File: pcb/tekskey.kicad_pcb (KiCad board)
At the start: 2 copper layers, 128.6 x 128.6 mm, 124 parts, among them J1 Conn_01x08, J2 Conn_01x08, SW0 MX_SW_HS, SW1 MX_SW_HS, SW10 MX_SW_HS, SW11 MX_SW_HS, SW12 MX_SW_HS, SW13 MX_SW_HS, SW14 MX_SW_HS, SW15 MX_SW_HS, SW1B1 MX_SW_HS, SW2 MX_SW_HS, SW20 MX_SW_HS, SW21 MX_SW_HS, SW22 MX_SW_HS, SW23 MX_SW_HS, SW24 MX_SW_HS, SW25 MX_SW_HS, SW2B1 MX_SW_HS, SW3 MX_SW_HS, SW30 MX_SW_HS, SW31 MX_SW_HS, SW32 MX_SW_HS, SW33 MX_SW_HS, SW34 MX_SW_HS, SW35 MX_SW_HS, SW3B1 MX_SW_HS, SW4 MX_SW_HS, SW40 MX_SW_HS, SW41 MX_SW_HS, SW42 MX_SW_HS, SW43 MX_SW_HS, SW44 MX_SW_HS, SW45 MX_SW_HS, SW4B1 MX_SW_HS, SW5 MX_SW_HS, SW50 MX_SW_HS, SW51 MX_SW_HS, SW51B1 MX_SW_HS, SW52 MX_SW_HS, SW53 MX_SW_HS, SW54 MX_SW_HS, SW55 MX_SW_HS, SW55B1 MX_SW_HS, SW5B1 MX_SW_HS

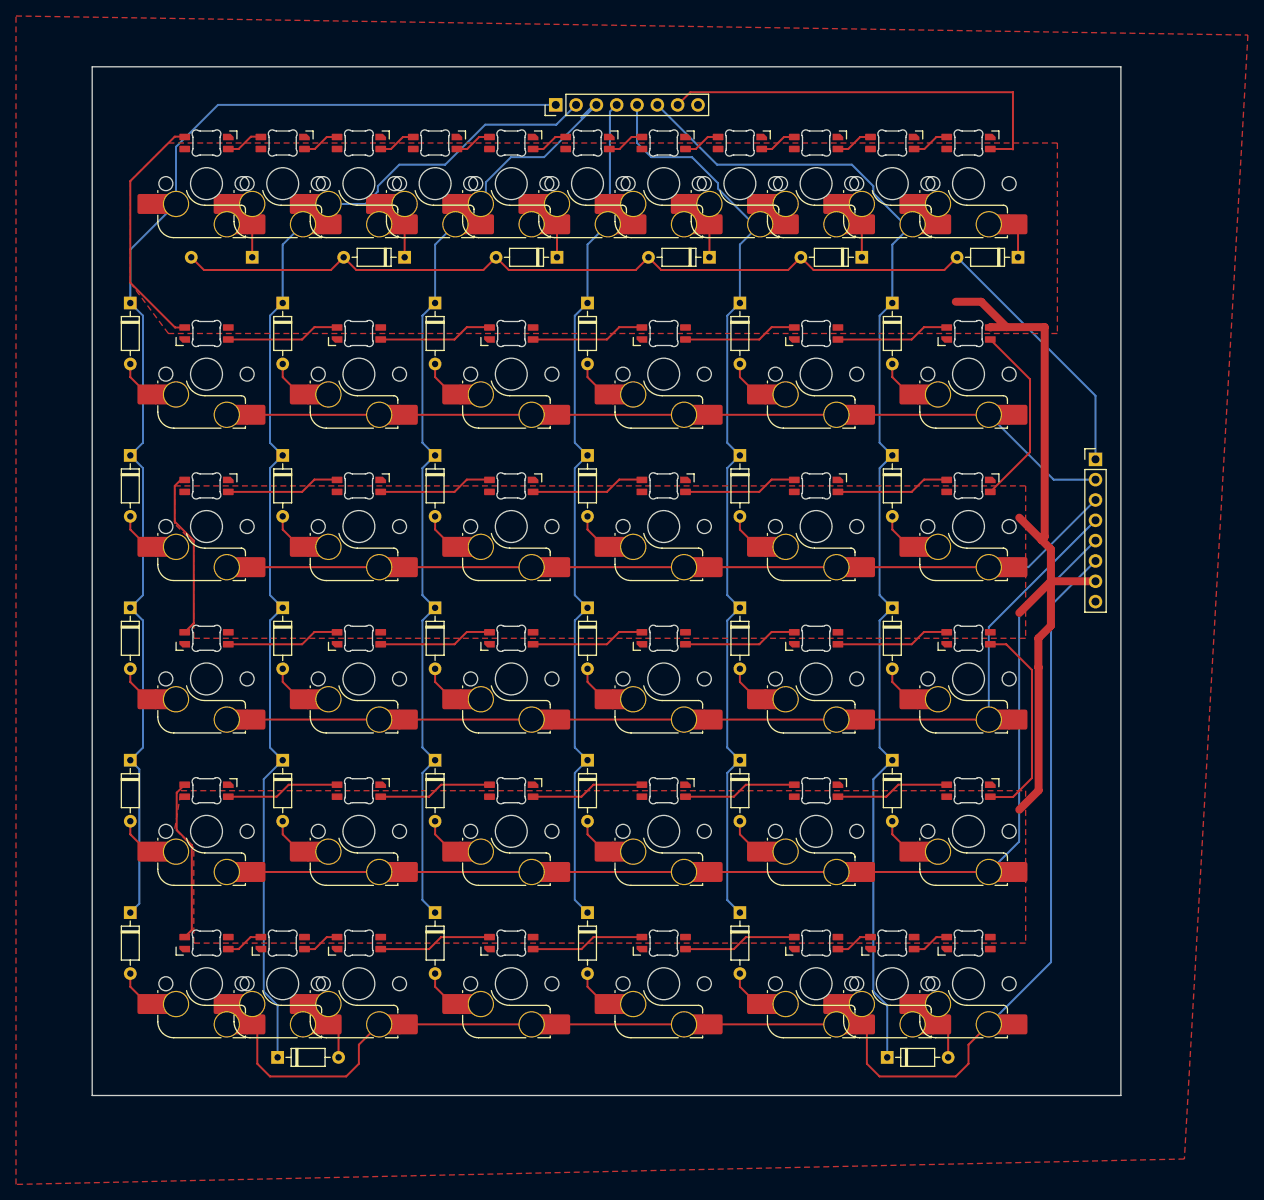
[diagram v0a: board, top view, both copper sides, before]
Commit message: wip
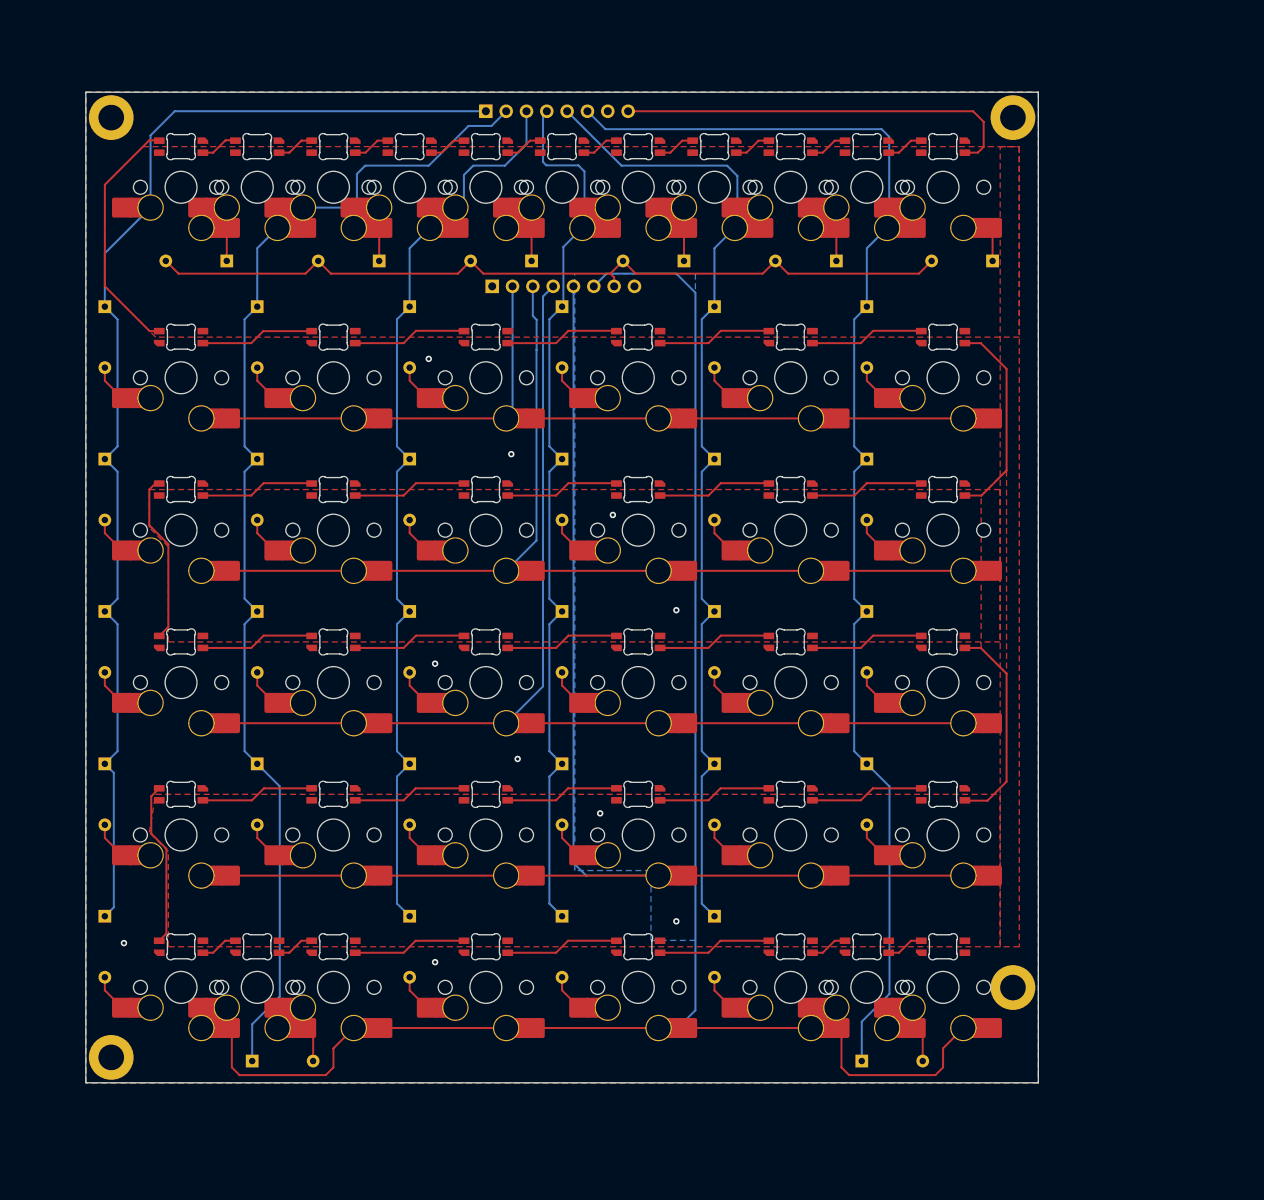
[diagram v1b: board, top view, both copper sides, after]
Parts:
- added J3: Conn_01x01_Male, MountingHole:MountingHole_3.2mm_M3_DIN965_Pad, F.Cu at (148.4, 30.2)
- added J4: Conn_01x01_Male, MountingHole:MountingHole_3.2mm_M3_DIN965_Pad, F.Cu at (35.7, 147.6)
- added J5: Conn_01x01_Male, MountingHole:MountingHole_3.2mm_M3_DIN965_Pad, F.Cu at (35.7, 30.2)
- added J6: Conn_01x01_Male, MountingHole:MountingHole_3.2mm_M3_DIN965_Pad, F.Cu at (148.4, 138.9)
- D1, D10, D11, D12, D13, D14, D15, D16, D17, D18, D19, D2, D20, D21, D22, D23, D24, D25, D26, D27, D28, D29, D3, D30, D31, D32, D33, D34, D35, D36, D4, D5, D6, D7, D8, D9: footprint Diode_THT:D_DO-35_SOD27_P7.62mm_Horizontal -> custom:D_DO-35_SOD27_P7.62mm_Horizontal_NoSilk
- moved J1 78.5 mm to (83.3, 51.3), turned to 90 degrees
- moved J2 8.77 mm to (82.5, 29.4)
- moved D13 3.21 mm to (73.0, 91.9)
- moved D18 3.21 mm to (130.2, 91.9)
- moved D21 3.21 mm to (73.0, 110.9)
- moved D24 3.21 mm to (130.2, 110.9)
- moved D27 3.21 mm to (73.0, 130.0)
- moved D30 3.21 mm to (129.5, 148.1)
- moved LED33 3.21 mm to (101.6, 95.7)
- moved LED34 3.21 mm to (120.6, 95.7)
- moved LED35 3.21 mm to (139.7, 95.7)
- moved LED43 3.21 mm to (101.6, 114.8)
- moved LED44 3.21 mm to (120.6, 114.8)
- moved LED45 3.21 mm to (139.7, 114.8)
- moved LED53 3.21 mm to (101.6, 133.8)
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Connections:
- J1 pad 1: row0 -> GND
- J1 pad 7: +5V -> row0
- J1 pad 8: GND -> +5V
- J2 pad 7: LEDIN -> GND
- J2 pad 8: unconnected-(J2-Pad8) -> LEDIN
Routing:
- net +5V: track 92.2 -> 0.00 mm, vias 0 -> 4
- net row5: track 172.2 -> 224.4 mm
- net row4: track 140.4 -> 176.9 mm
- net row0: track 134.7 -> 104.1 mm
- net row3: track 125.7 -> 152.3 mm
- net row2: track 112.1 -> 132.6 mm
- net col5: track 153.0 -> 169.1 mm
- net col4: track 120.7 -> 130.3 mm
- net col0: track 152.6 -> 148.0 mm
- net Net-(D32-Pad1): track 7.42 -> 11.0 mm
- net Net-(D35-Pad1): track 7.42 -> 11.0 mm
- net Net-(D34-Pad1): track 7.42 -> 11.0 mm
- net Net-(D26-Pad2): track 5.36 -> 8.96 mm
- net Net-(D33-Pad1): track 7.42 -> 11.0 mm
- net Net-(D30-Pad2): track 6.82 -> 10.4 mm
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- added copper zone on B.Cu, net +5V
- added copper zone on B.Cu, net GND
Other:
- board size 128.6 x 128.6 mm -> 119.1 x 123.8 mm
